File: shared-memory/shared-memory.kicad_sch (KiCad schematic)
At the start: 6 parts, among them U1 74HC00, U2 CH32V003FxPx, U3 CH32V003FxPx, U5 74LVC125, U6 74LVC125

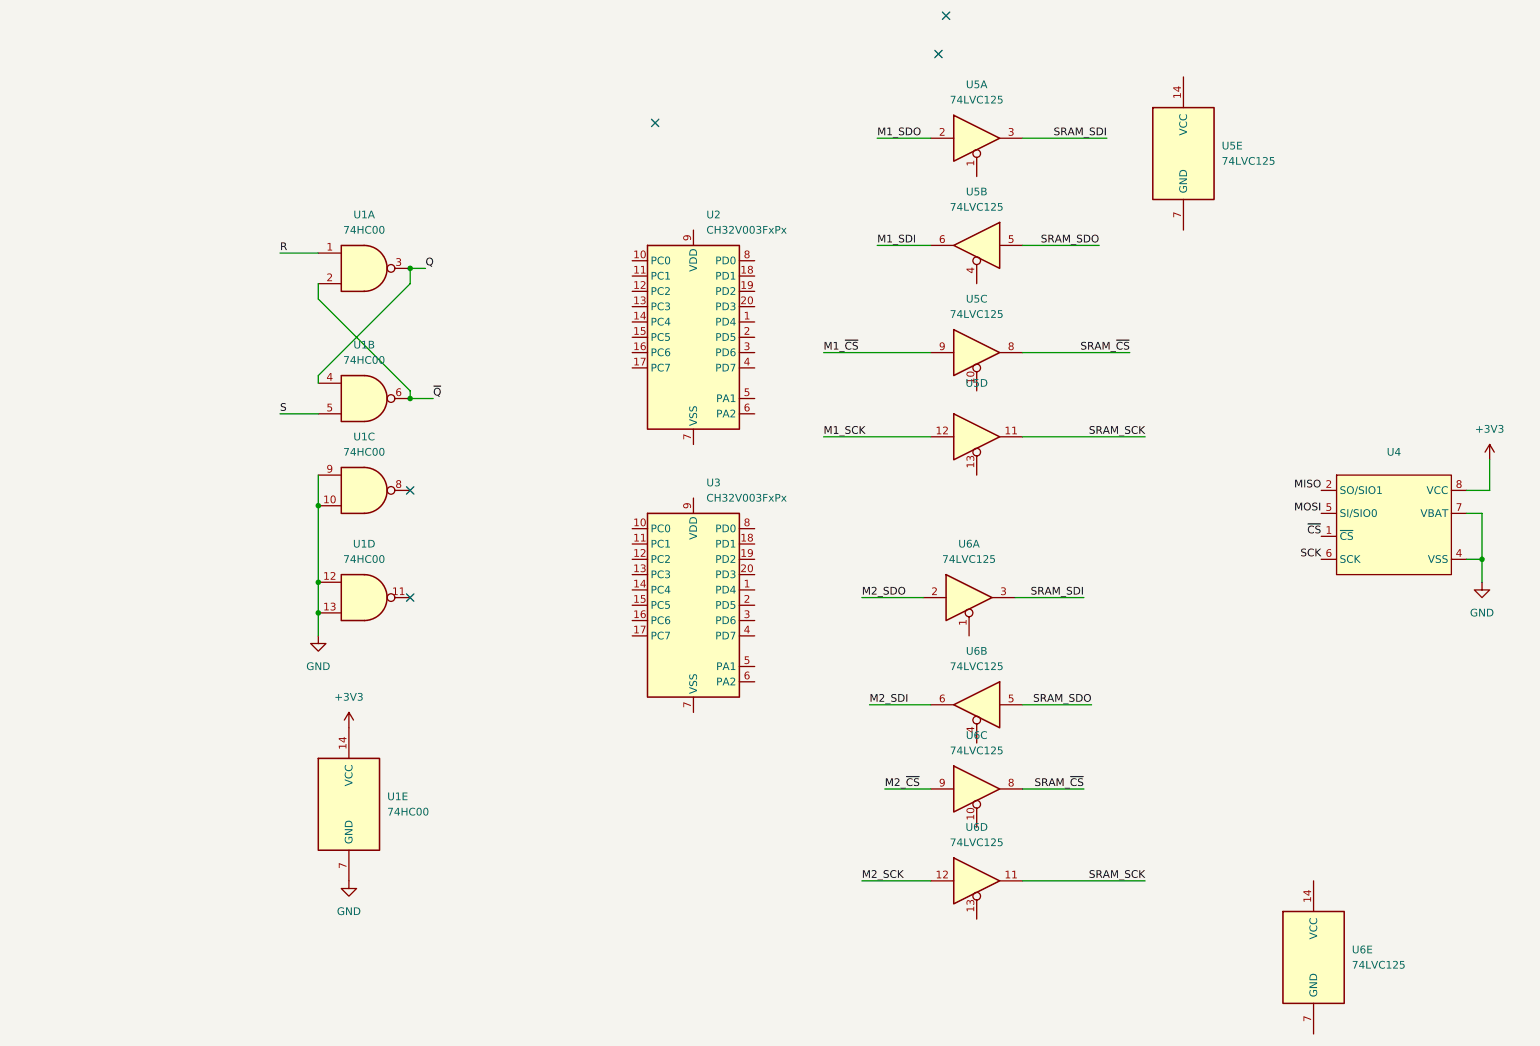
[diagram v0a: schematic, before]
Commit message: imprved the schematic
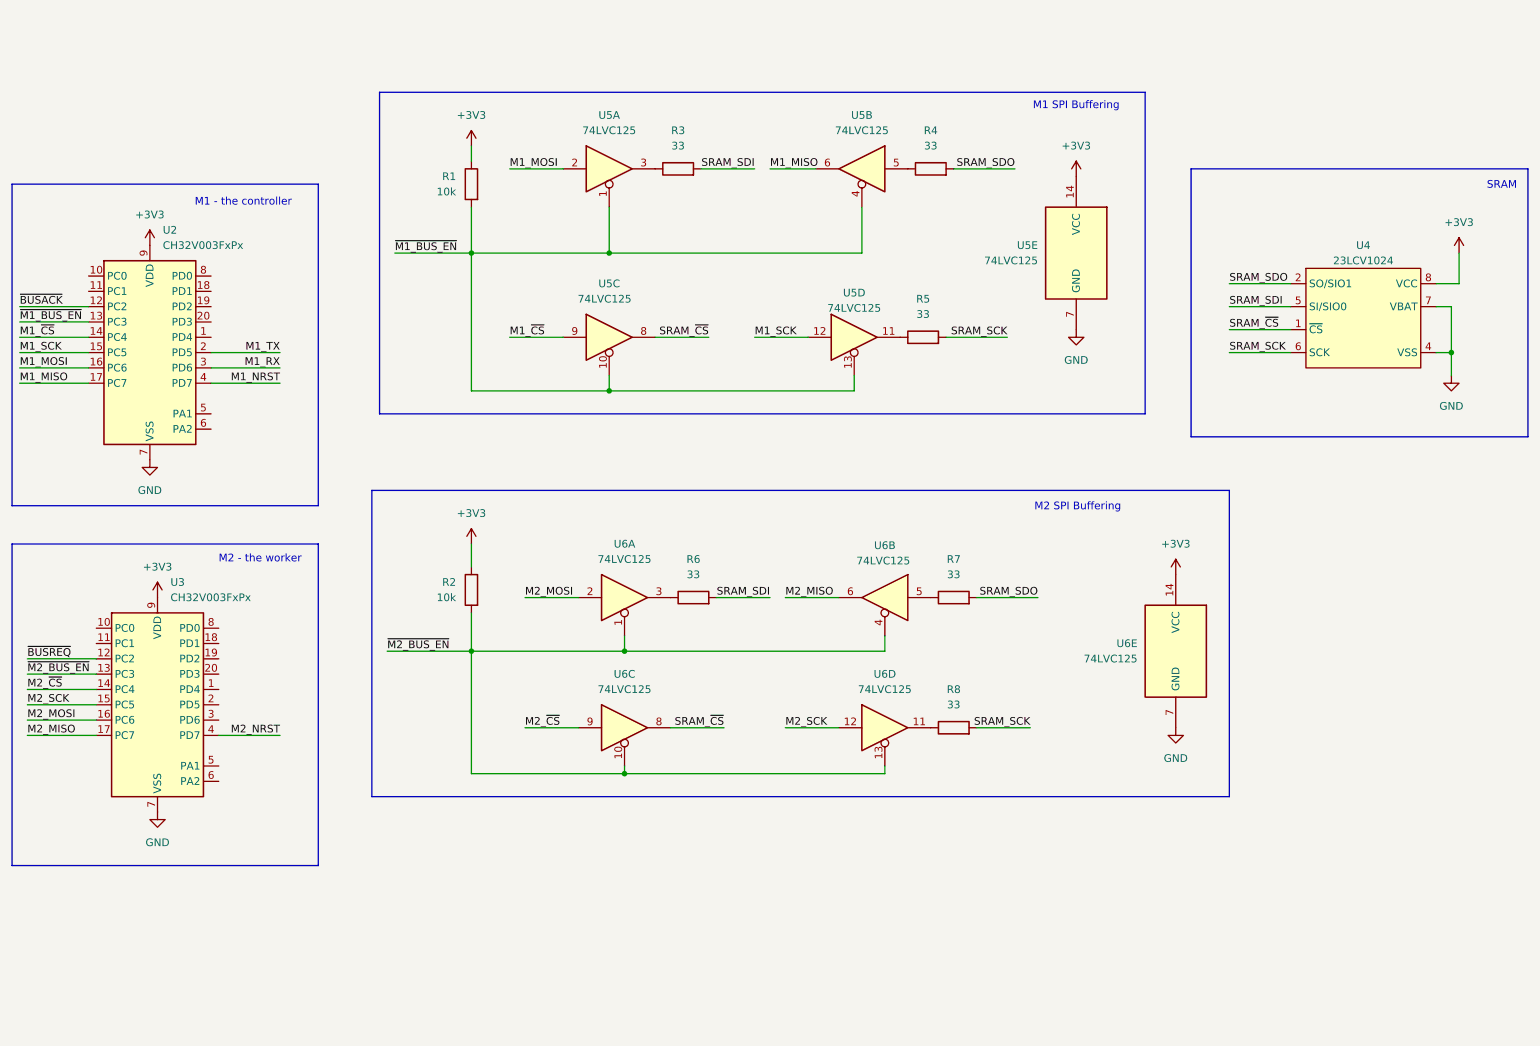
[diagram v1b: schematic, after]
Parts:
- removed U1: 74HC00, symbol 74xx:74HC00
- added R1, R2: 10k, symbol Device:R
- added R3, R4, R5, R6, R7, R8: 33, symbol Device:R
- U4: value ~ -> 23LCV1024
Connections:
- net M1_SDI is gone; now on net M1_MISO: U5.6
- net M1_SDO is gone; now on net M1_MOSI: U5.2
- net M2_SDI is gone; now on net M2_MISO: U6.6
- net M2_SDO is gone; now on net M2_MOSI: U6.2
- net MISO is gone; now on net SRAM_SDO: U4.2 (SO/SIO1)
- net MOSI is gone; now on net SRAM_SDI: U4.5 (SI/SIO0)
- net SCK is gone; now on net SRAM_SCK: U4.6 (SCK)
- net ~{CS} is gone; now on net SRAM_~{CS}: U4.1 (~{CS})
- net +3V3: now also U2.9 (VDD), U3.9 (VDD), U5.14 (VCC), U6.14 (VCC), R1.1, R2.1
- net GND: now also U2.7 (VSS), U3.7 (VSS), U5.7 (GND), U6.7 (GND)
- net M1_SCK: now also U2.15 (PC5)
- net M1_~{CS}: now also U2.14 (PC4)
- net M2_SCK: now also U3.15 (PC5)
- net M2_~{CS}: now also U3.14 (PC4)
- net SRAM_SCK: now also R5.2, R8.2; no longer U5.11, U6.11
- net SRAM_SDI: now also R3.2, R6.2; no longer U5.3, U6.3
- net SRAM_SDO: now also R4.2, R7.2; no longer U5.5, U6.5
- net ~{M1_BUS_EN}: now reaches U5.13
- net ~{M1_BUS_EN}: now also U2.13 (PC3), U5.1, U5.10, U5.4, R1.2
- net ~{BUSACK}: now reaches U2.12 (PC2)
- net M1_MOSI: now reaches U2.16 (PC6)
- net M1_MISO: now reaches U2.17 (PC7)
- net M1_TX: now reaches U2.2 (PD5)
- net M1_RX: now reaches U2.3 (PD6)
- net M1_NRST: now reaches U2.4 (PD7)
- net ~{BUSREQ}: now reaches U3.12 (PC2)
- net ~{M2_BUS_EN}: now reaches U3.13 (PC3)
- net ~{M2_BUS_EN}: now also U6.1, U6.10, U6.13, U6.4, R2.2
- net M2_MOSI: now reaches U3.16 (PC6)
- net M2_MISO: now reaches U3.17 (PC7)
- net M2_NRST: now reaches U3.4 (PD7)
- new net: R7.1, U6.5
- new net: R5.1, U5.11
- new net: R6.1, U6.3
- new net: R3.1, U5.3
- new net: R8.1, U6.11
- new net: R4.1, U5.5
- no-connect marks 5 -> 0
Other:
- note added: "M1 - the controller"
- note added: "M1 SPI Buffering"
- note added: "M2 - the worker"
- note added: "M2 SPI Buffering"
- note added: "SRAM"
- moved on the sheet: U2, U3, U4, U5A, U5B, U5C, U5E, U6A, U6B, U6C, U6D, U6E
